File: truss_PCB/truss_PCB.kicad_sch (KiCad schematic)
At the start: 8 parts, among them J1 XT60_60A_male, J2 LimitSwitch, J3 Servo, J4 Truss Connection

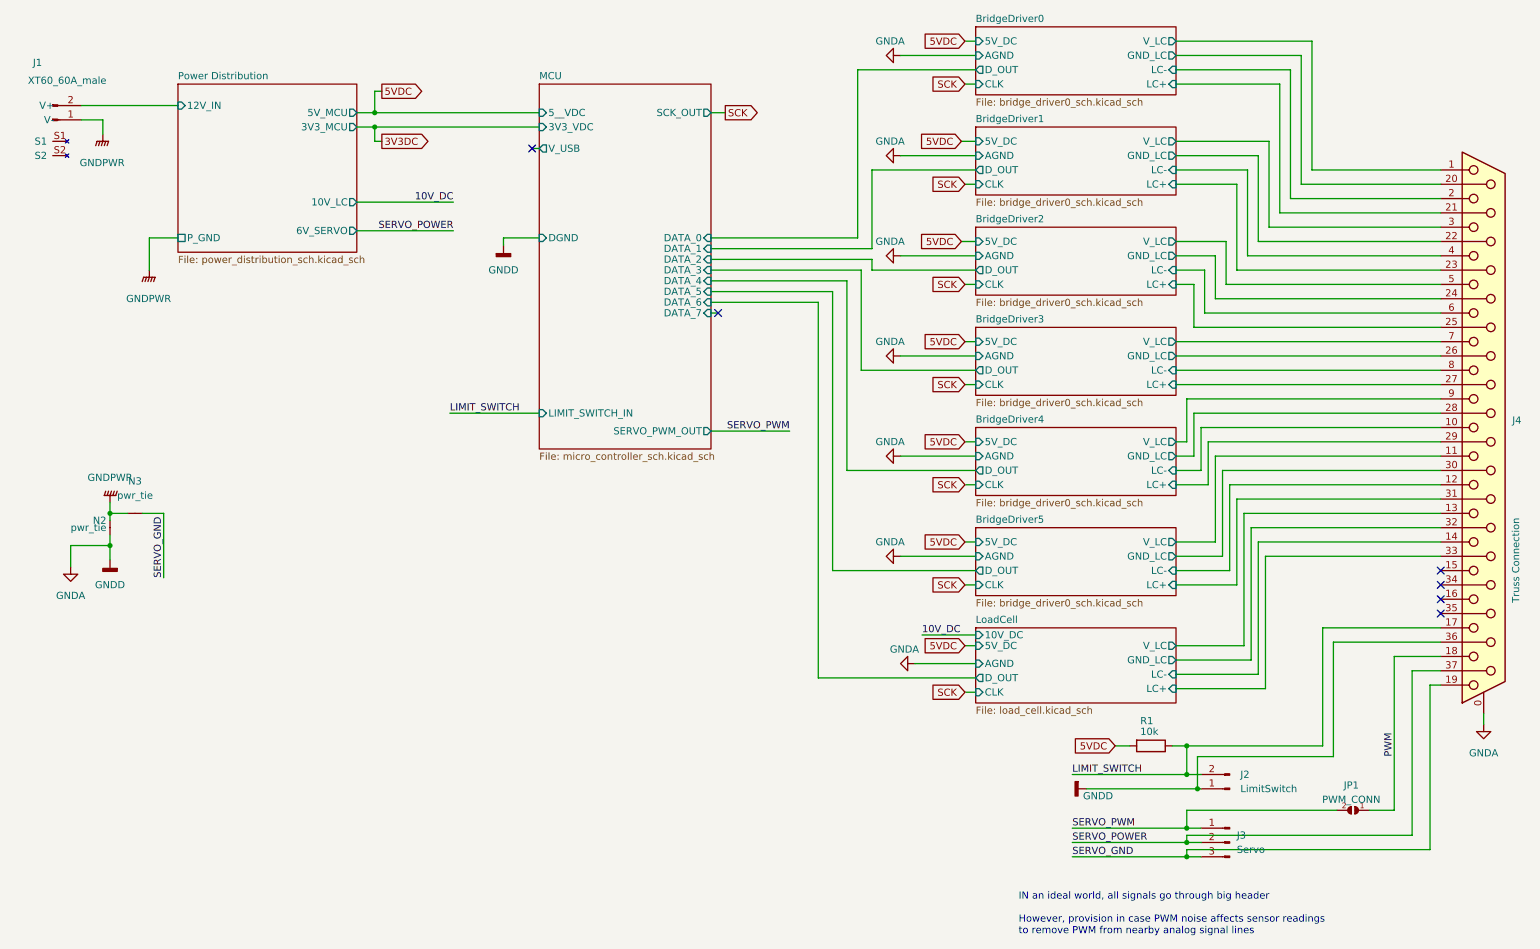
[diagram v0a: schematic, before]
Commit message: updating truss PCB
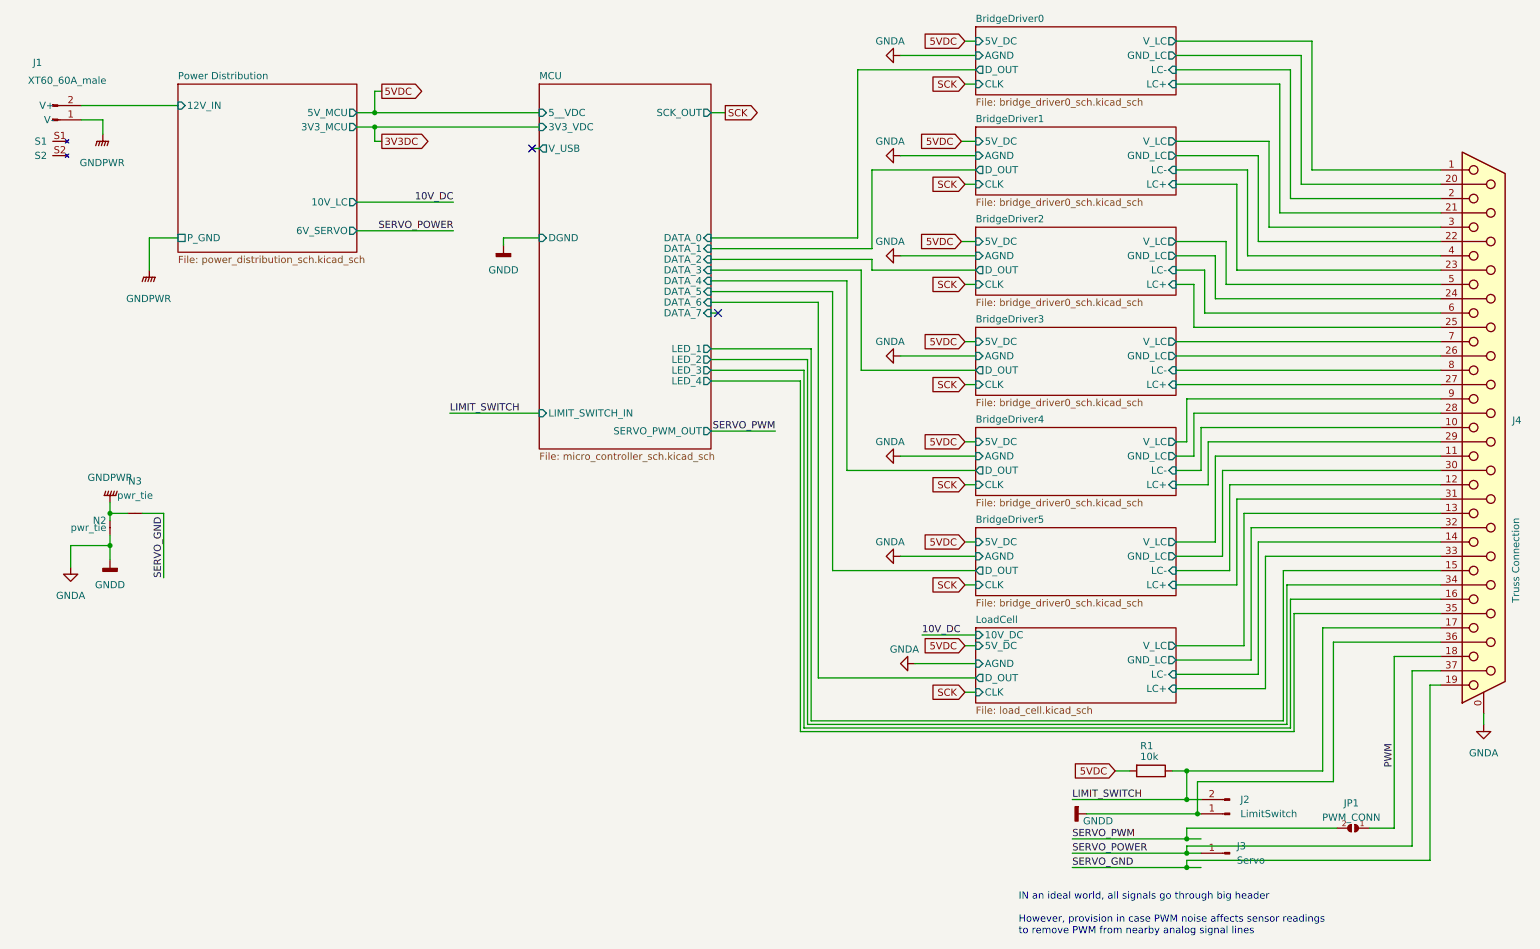
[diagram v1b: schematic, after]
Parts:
- J3: symbol Connector:Conn_01x03_Male -> Connector:Conn_01x01_Male
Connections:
- net SERVO_GND: no longer J3.3 (Pin_3)
- net SERVO_POWER: now also J3.1 (Pin_1); no longer J3.2 (Pin_2)
- net SERVO_PWM: no longer J3.1 (Pin_1)
- net MCU/LED_1: now reaches J4.15
- net MCU/LED_3: now reaches J4.16
- net MCU/LED_2: now reaches J4.34
- net MCU/LED_4: now reaches J4.35
- no-connect marks 6 -> 2
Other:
- sheet MCU ports: added LED_1, LED_2, LED_3, LED_4; removed none
- moved on the sheet: J2, JP1, R1
